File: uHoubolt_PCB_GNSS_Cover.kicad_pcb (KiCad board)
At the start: 2 copper layers, 85.8 x 85.8 mm, 5 parts

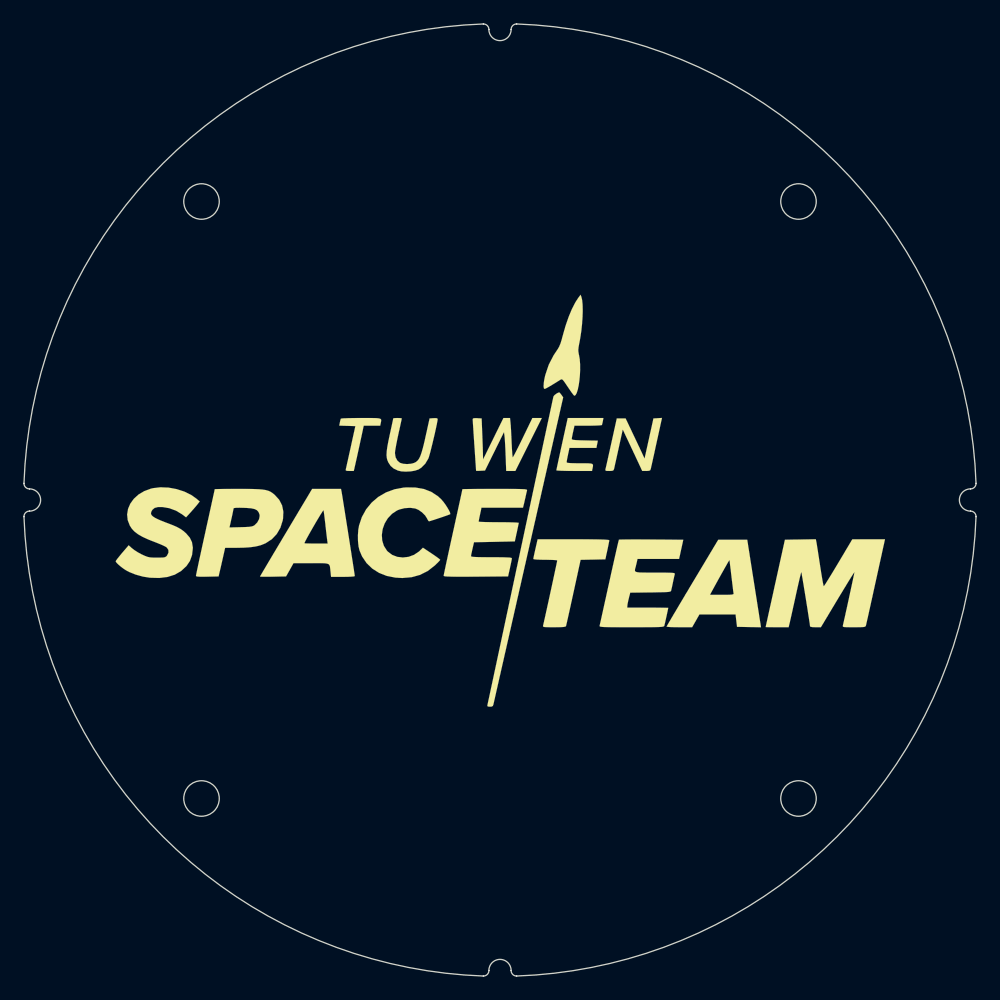
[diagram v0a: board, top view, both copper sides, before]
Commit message: Cover
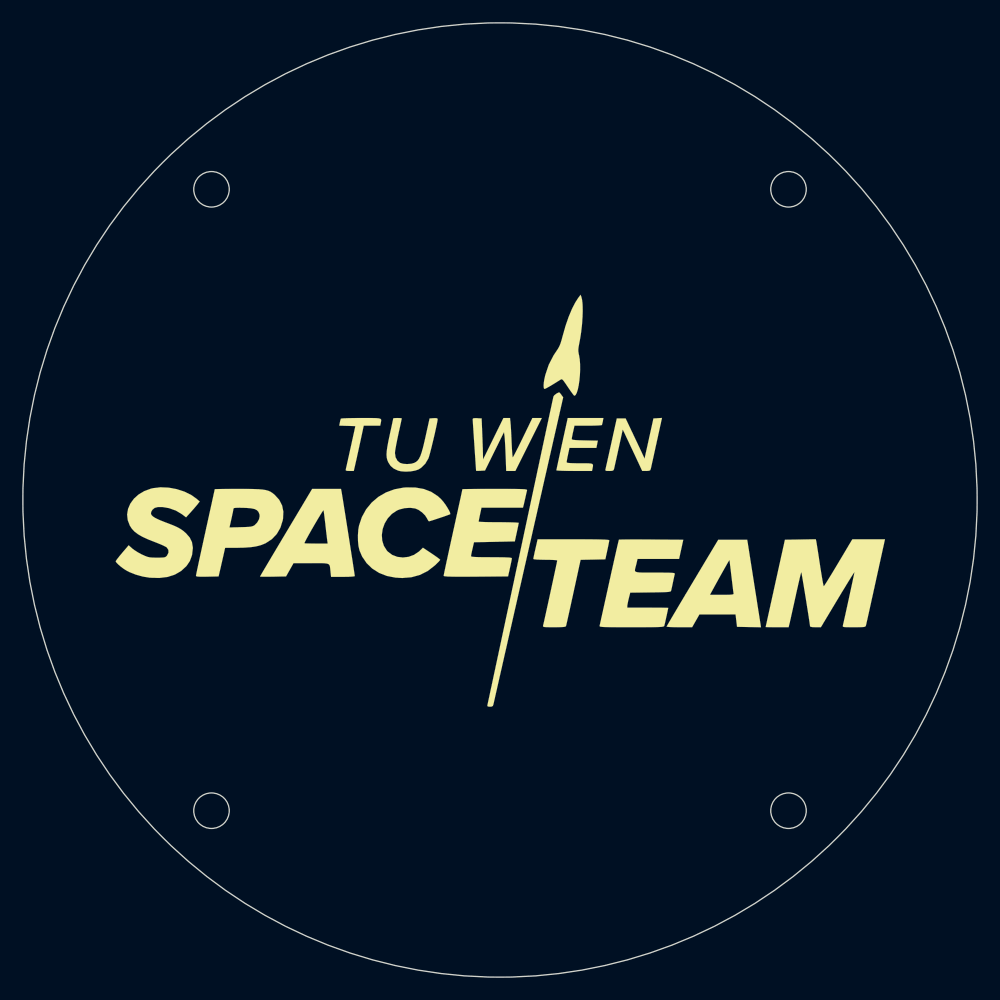
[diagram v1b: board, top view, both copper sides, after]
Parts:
- moved REF** 1.42 mm to (124.0, 72.0)
- moved REF** 1.42 mm to (176.0, 72.0)
- moved REF** 1.42 mm to (176.0, 128.0)
- moved REF** 1.42 mm to (124.0, 128.0)
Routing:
- net (no net): track 0.00 -> 625.3 mm
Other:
- board size 85.8 x 85.8 mm -> 86 x 86 mm
- net class Default removed
- board text added: "JLCJLCJLCJLC"
